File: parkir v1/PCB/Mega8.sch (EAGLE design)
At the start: 18 parts, among them K1 ZF112, Q1 BC447, Q2 BC448

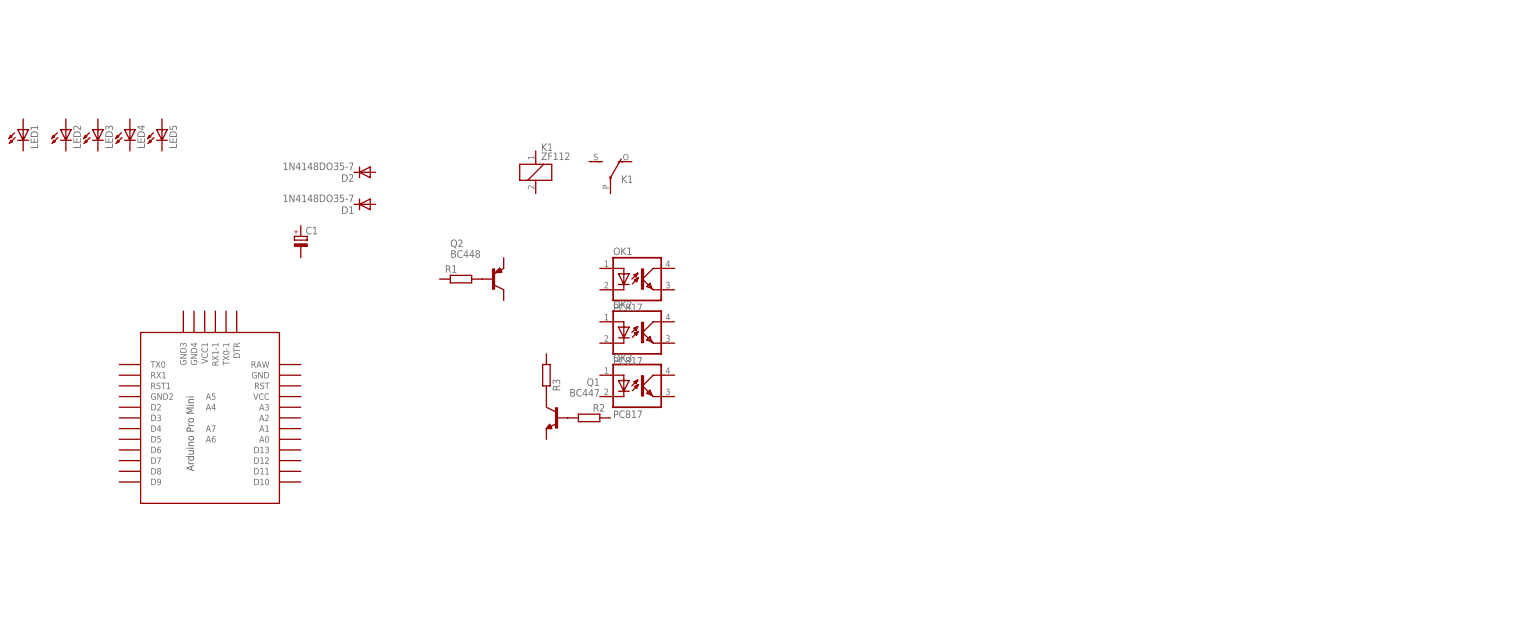
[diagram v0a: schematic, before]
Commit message: relayout
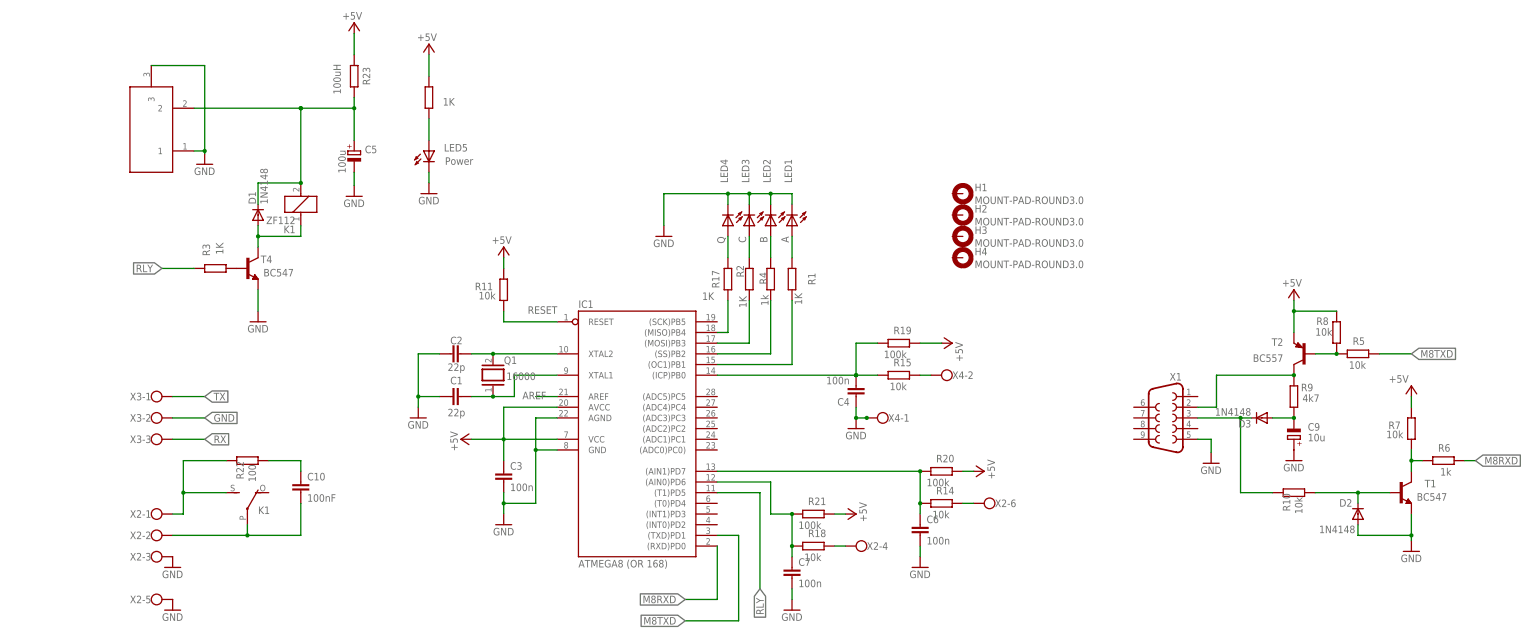
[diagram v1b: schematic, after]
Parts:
- removed OK1, OK2, OK3: PC817, optocoupler:PC817
- removed Q2: BC448, transistor-pnp:BC448
- removed U$1: PRO-MINI-2, arduino_clone:PRO-MINI-2
- added C10: 100nF, rcl:C-EU102-043X133
- added C2: 22p, rcl:C-EU050-025X075
- added C3, C4, C6, C7: 100n, rcl:C-EU050-025X075
- added C5: 100u, rcl:CPOL-EUE3.5-8
- added C9: 10u, rcl:CPOL-EUE5-6
- added D3: 1N4148, diode:1N4148
- added DC1: DC21MMX, powersupply:DC21MMX
- added H1, H2, H3, H4: MOUNT-PAD-ROUND3.0, holes:MOUNT-PAD-ROUND3.0
- added IC1: ATMEGA8 (OR 168), atmel:AT90S4433P
- added R10, R11, R14, R15, R18, R5, R7, R8: 10k, rcl:R-EU_0207/10
- added R16, R17: 1K, rcl:R-EU_0207/10
- added R19, R20, R21: 100k, rcl:R-EU_0207/10
- added R22: 100, rcl:R-EU_0207/10
- added R23: 100uH, rcl:R-EU_0207/10
- added R4, R6: 1k, rcl:R-EU_0207/10
- added R9: 4k7, rcl:R-EU_0207/10
- added T1, T4: BC547, transistor:BC547
- added T2: BC557, transistor:BC557B-PNP-TO92-EBC
- added X1: (no value), con-subd:F09H
- added X2: (no value), con-wago-500:W237-6
- added X3: (no value), con-wago-500:W237-103
- added X4: (no value), con-wago-500:W237-102
- C1: value (none) -> 22p; device rcl:CPOL-EUE5-6 -> rcl:C-EU050-025X075
- D1, D2: value 1N4148DO35-7 -> 1N4148; device diode:1N4148DO35-7 -> diode:1N4148
- LED1: value (none) -> A; device led:LED5MM -> led:LED3MM
- LED2: value (none) -> B; device led:LED5MM -> led:LED3MM
- LED3: value (none) -> C; device led:LED5MM -> led:LED3MM
- LED4: value (none) -> Q; device led:LED5MM -> led:LED3MM
- LED5: value (none) -> Power; device led:LED5MM -> led:LED3MM
- Q1: value BC447 -> 16000; device transistor-npn:BC447 -> special:XTAL
- R1, R2, R3: value (none) -> 1K; device rcl:R-EU_0207/7 -> rcl:R-EU_0207/10
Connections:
- new net +5V: C3.1, IC1.AVCC, IC1.VCC, R11.2, R16.2, R19.1, R20.1, R21.1, R23.2, R7.2, R8.1, T2.E
- new net AREF: IC1.AREF
- new net GND: C1.1, C2.1, C3.2, C4.1, C5.-, C6.2, C7.2, C9.+, D2.A, DC1.1, DC1.3, IC1.AGND, IC1.GND, LED1.C, LED2.C, LED3.C, LED4.C, LED5.C, T1.E, T4.E, X1.5, X2-3.KL, X2-5.KL, X3-2.KL, X4-1.KL
- new net M8RXD: IC1.(RXD)PD0, R6.1
- new net M8TXD: IC1.(TXD)PD1, R5.1
- new net N$13: C4.2, IC1.(ICP)PB0, R15.2, R19.2
- new net N$14: C6.1, IC1.(AIN1)PD7, R14.2, R20.2
- new net N$15: R14.1, X2-6.KL
- new net N$16: IC1.(OC1)PB1, R1.2
- new net N$17: IC1.(SS)PB2, R4.2
- new net N$18: IC1.(MOSI)PB3, R2.2
- new net N$19: LED5.A, R16.1
- new net N$20: C7.1, IC1.(AIN0)PD6, R18.2, R21.2
- new net N$21: LED4.A, R17.1
- new net N$22: IC1.(MISO)PB4, R17.2
- new net N$23: R15.1, X4-2.KL
- new net N$26: R6.2, R7.1, T1.C
- new net N$27: R5.2, R8.2, T2.B
- new net N$28: C10.1, R22.1
- new net N$29: D2.C, R10.1, T1.B
- new net N$30: C5.+, D1.C, DC1.2, K11.2, R23.1
- new net N$32: LED3.A, R2.1
- new net N$33: LED1.A, R1.1
- new net N$4: D1.A, K11.1, T4.C
- new net N$5: R18.1, X2-4.KL
- new net N$6: C1.2, IC1.XTAL1, Q1.1
- new net N$7: C2.2, IC1.XTAL2, Q1.2
- new net N$8: K12.S, R22.2, X2-1.KL
- new net N$9: C10.2, K12.P, X2-2.KL
- new net RESET: IC1.RESET, R11.1
- new net RLY: IC1.(T1)PD5, R3.2
- new net RX: D3.C, R10.2, X1.3, X3-3.KL
- new net TX: R9.2, T2.C, X1.2, X3-1.KL
- net N$1: now also R3.1, T4.B; no longer Q2.B, R1.2
- net N$2: now also C9.-, D3.A, R9.1; no longer Q1.B, R2.2
- net N$3: now also LED2.A, R4.1; no longer Q1.C, R3.1
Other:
- moved on the sheet: D1, D2, K1, LED1, LED2, LED3, LED4, LED5, R1, R2, R3
